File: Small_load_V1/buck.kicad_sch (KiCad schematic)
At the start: 16 parts, among them J11 Input, J14 Jack-DC, Q4 HYG025N06LS1C2, Q6 HYG025N06LS1C2, U6 LM5109BMA

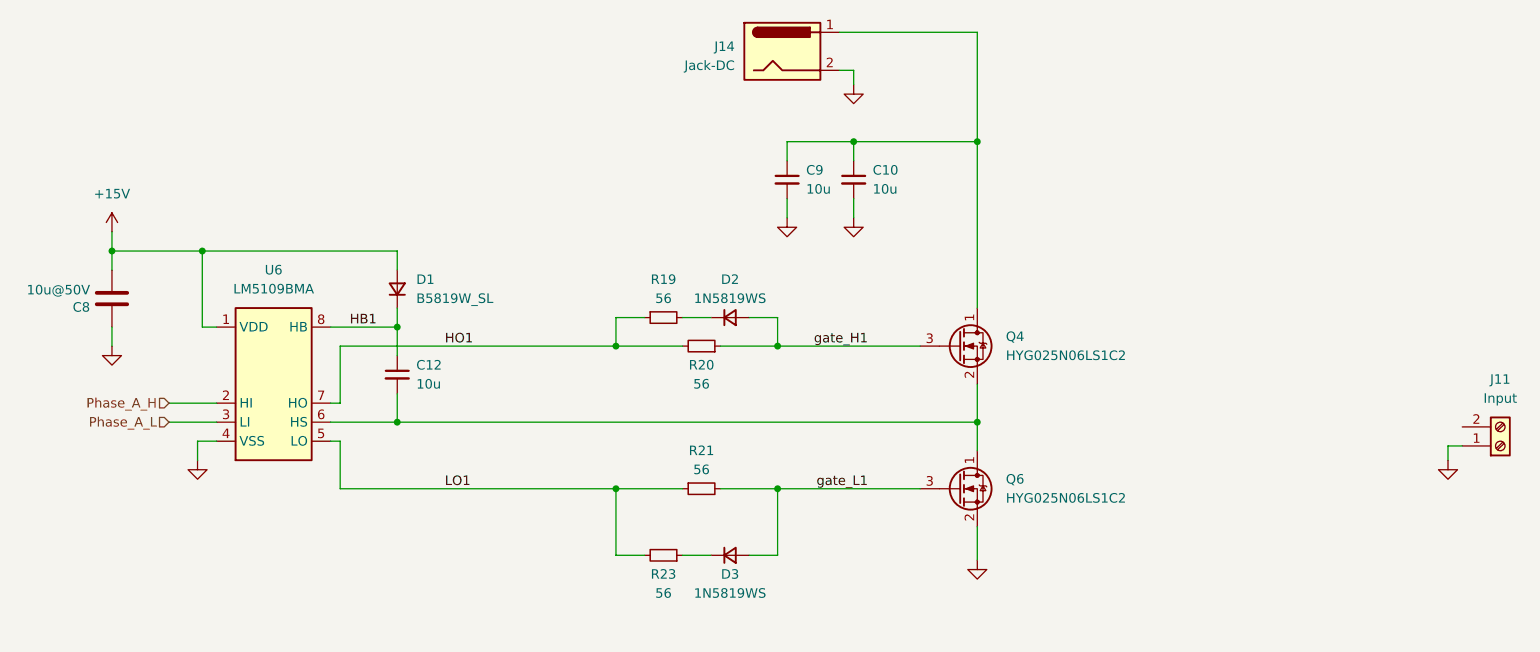
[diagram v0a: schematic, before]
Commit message: g
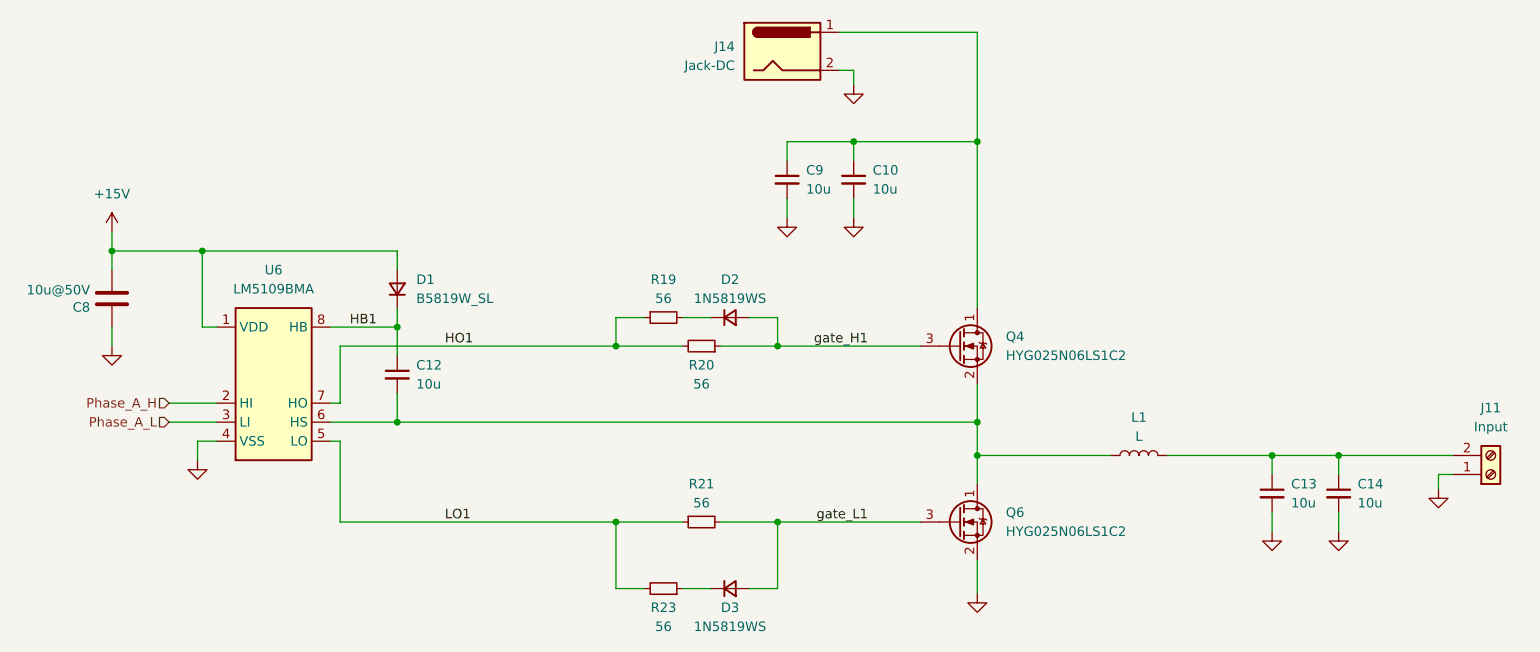
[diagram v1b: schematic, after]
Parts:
- added C13, C14: 10u, Capacitor_SMD:C_1206_3216Metric, symbol Device:C_Small
- added L1: L, symbol Device:L
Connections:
- net GND: now also C13.2, C14.2
- net at C12.2, Q4.2 (S), Q6.1 (D)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: now also L1.1
- net at J11.2 (Pin_2): now also C13.1, C14.1, L1.2
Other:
- moved on the sheet: D3, J11, Q6, R21, R23
